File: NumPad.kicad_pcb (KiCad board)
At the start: 2 copper layers, 60.7 x 98.9 mm, 112 parts, among them J1 Micro_SD_Card_Det, J2 OLED1, J3 OLED2, J4 Conn_01x05_Female, SW1 SW_SPST, SW10 SW_SPST, SW11 SW_SPST, SW12 SW_SPST, SW13 SW_SPST, SW14 SW_SPST, SW15 SW_SPST, SW16 SW_SPST, SW17 SW_SPST, SW18 SW_SPST, SW19 SW_SPST, SW2 SW_SPST, SW20 SW_SPST, SW21 SW_SPST, SW22 SW_SPST, SW23 SW_SPST, SW24 SW_SPST, SW25 SW_BUTTONRESET, SW26 SW_BUTTON2, SW27 SW_BUTTON1, SW28 SW_BOOT0, SW29 Rotary_Encoder_Switch, SW3 SW_SPST, SW4 SW_SPST, SW5 SW_SPST, SW6 SW_SPST, SW7 SW_SPST, SW8 SW_SPST, SW9 SW_SPST, U1 LM117_TO3, U2 STM32F072C8Tx, U3 74AHCT1G08

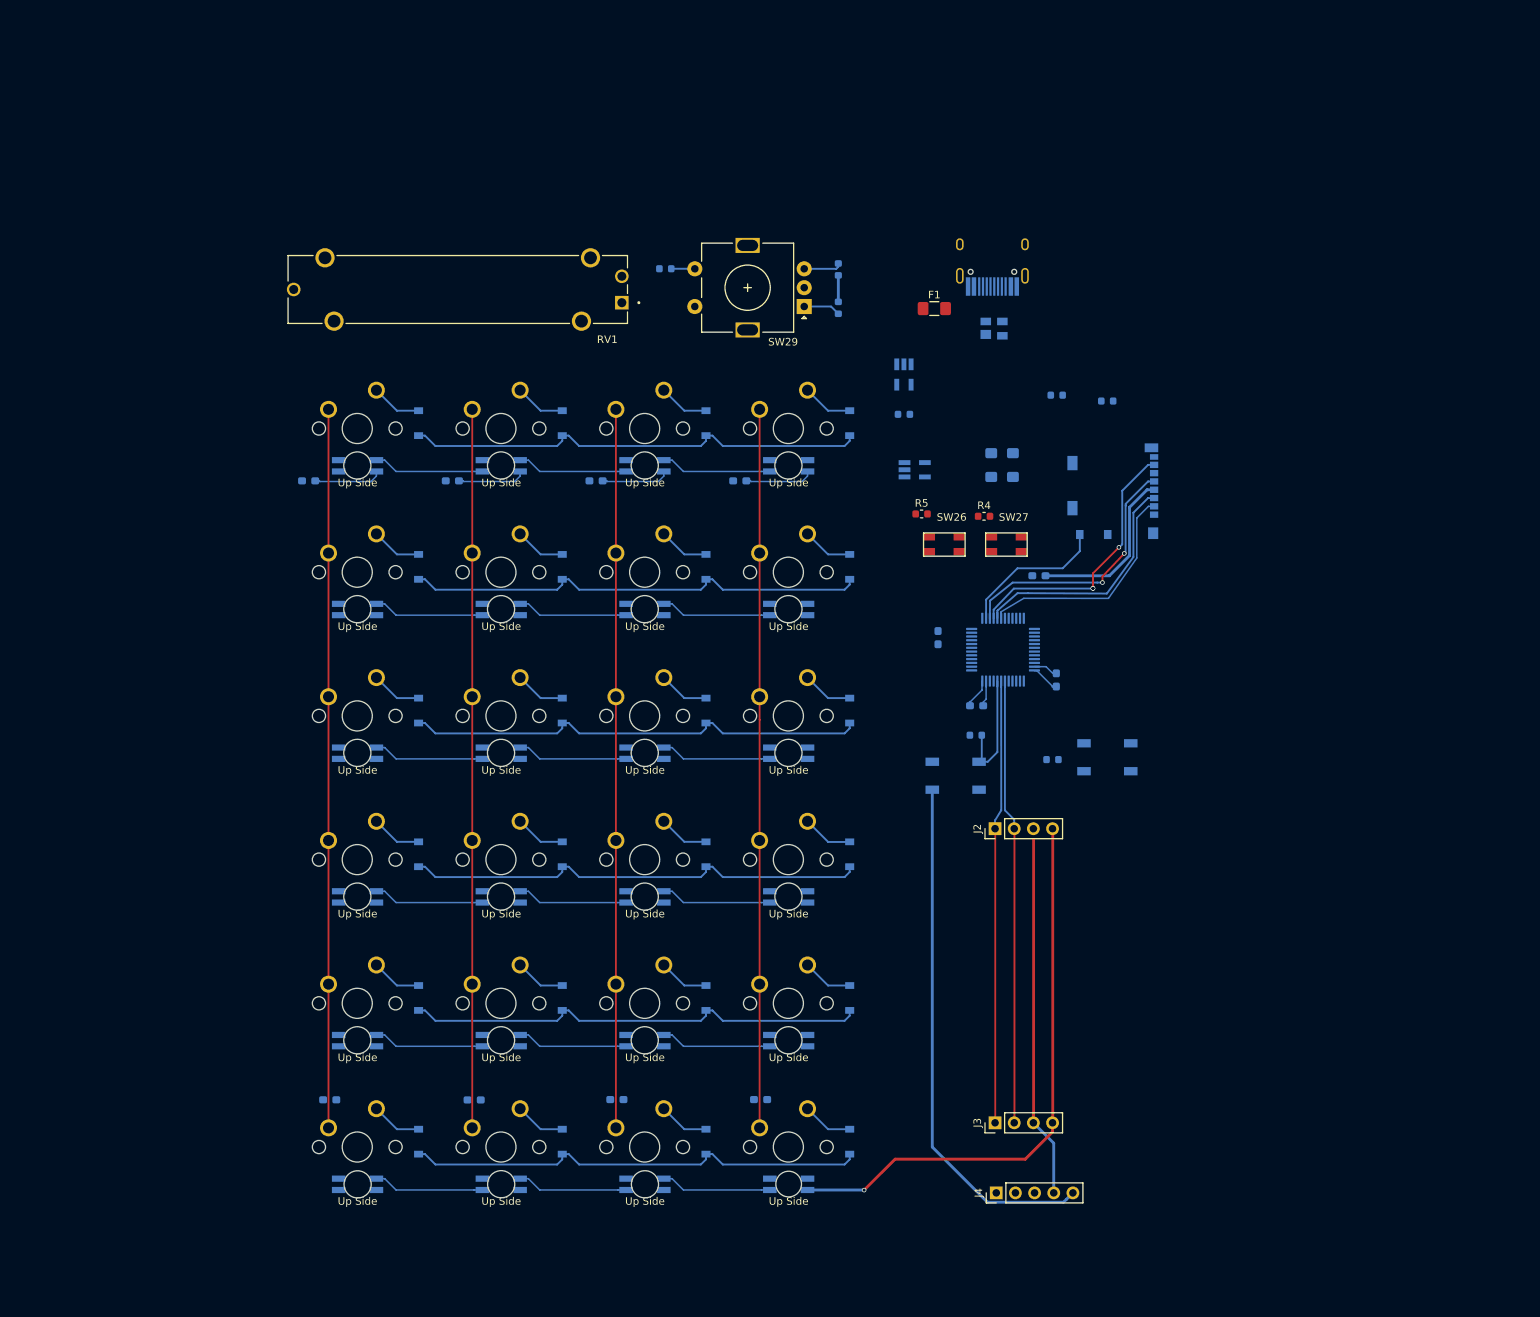
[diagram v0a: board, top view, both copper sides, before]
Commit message: update PCB
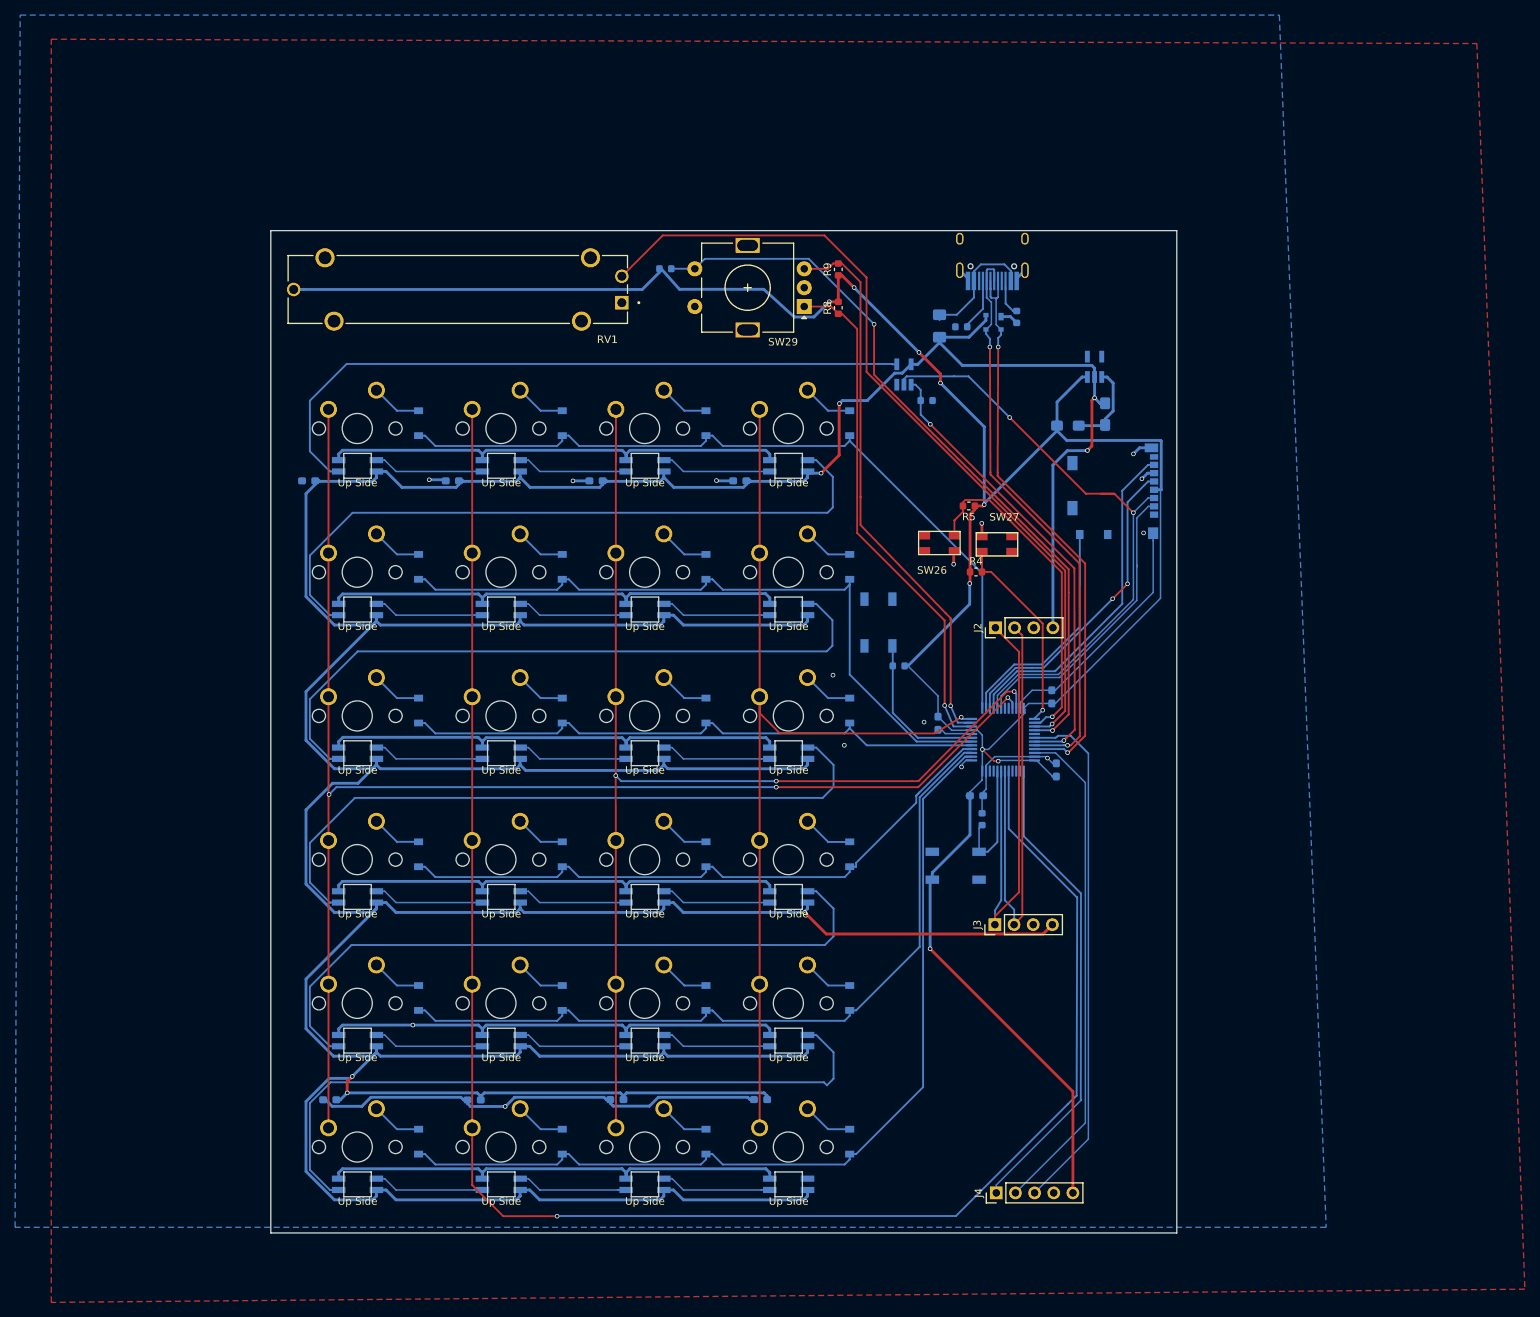
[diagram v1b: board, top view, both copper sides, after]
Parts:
- D1: footprint Package_TO_SOT_SMD:SOT-143 -> random-keyboard-parts:SOT143B
- F1: moved to B.Cu
- R8, R9: moved to F.Cu
- moved SW25 35.2 mm to (100.5, 102.8), turned to 90 degrees
- moved U1 27.5 mm to (129.1, 68.8), turned to 90 degrees
- moved J2 26.6 mm to (116.0, 103.4)
- moved J3 26.3 mm to (115.9, 142.8)
- moved R3 23.9 mm to (103.1, 108.5), turned to 180 degrees
- moved R1 21.7 mm to (111.4, 63.5)
- moved C4 16.1 mm to (123.4, 112.6), turned to 90 degrees
- moved C1 14.6 mm to (130.5, 75.1), turned to 270 degrees
- moved C5 11.9 mm to (124.0, 122.3)
- moved SW28 11.9 mm to (110.7, 135.0)
- moved U2 11.9 mm to (117.0, 118.3)
- moved C6 11.9 mm to (113.5, 125.7)
- moved R2 11.7 mm to (118.8, 62.2), turned to 90 degrees
- moved C3 11.3 mm to (108.3, 116.1)
- moved R6 11.2 mm to (114.2, 128.8), turned to 90 degrees
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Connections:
- R5 pad 2: Net-(R5-Pad2) -> BUT2
- SW26 pad 1: Net-(R5-Pad2) -> BUT2
- U2 pad 12: row4 -> col3
- U2 pad 13: Net-(R5-Pad2) -> row0
- U2 pad 25: POT_SLIDER -> BUT1
- U2 pad 26: Net-(U2-Pad26) -> BUT2
- U2 pad 27: Net-(U2-Pad27) -> POT_SLIDER
- U2 pad 28: Net-(U2-Pad28) -> ENC_SWITCH
- U2 pad 3: col3 -> row4
- U2 pad 38: BUT1 -> Net-(U2-Pad38)
- U2 pad 39: ENC_SWITCH -> Net-(U2-Pad39)
- U2 pad 4: row0 -> row3
- U2 pad 45: row3 -> Net-(U2-Pad45)
- U2 pad 5: row1 -> row2
- U2 pad 6: row2 -> row1
- U3 pad 5: VCC -> +5V
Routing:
- net +5V: track 112.1 -> 737.3 mm, vias 1 -> 7
- net GND: track 56.1 -> 528.2 mm, vias 0 -> 15
- net +3V3: track 103.6 -> 337.7 mm, vias 0 -> 9
- net col1: track 95.2 -> 238.1 mm, vias 0 -> 1
- net POT_SLIDER: track 0.00 -> 110.3 mm, vias 0 -> 1
- net col0: track 95.2 -> 192.2 mm, vias 0 -> 3
- net ENC_SWITCH: track 3.13 -> 98.9 mm, vias 0 -> 2
- net Net-(D31-Pad4): track 0.00 -> 92.8 mm
- net Net-(D26-Pad4): track 0.00 -> 91.5 mm
- net Net-(D27-Pad4): track 0.00 -> 90.5 mm
- net Net-(D30-Pad4): track 0.00 -> 90.4 mm
- net Net-(D29-Pad4): track 0.00 -> 90.0 mm
- net Net-(D28-Pad4): track 0.00 -> 90.0 mm
- net USB_DN: track 0.00 -> 76.7 mm, vias 0 -> 2
- net USB_DP: track 0.00 -> 76.0 mm, vias 0 -> 2
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- added copper zone on B.Cu, net GND
- added copper zone on F.Cu, net GND
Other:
- board size 60.7 x 98.9 mm -> 120.1 x 132.9 mm
